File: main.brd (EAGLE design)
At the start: 49.5 x 36.8 mm, 27 parts, among them IC1 FT232RL, U1 ATMEGA328P_TQFP, Y3 16MHz

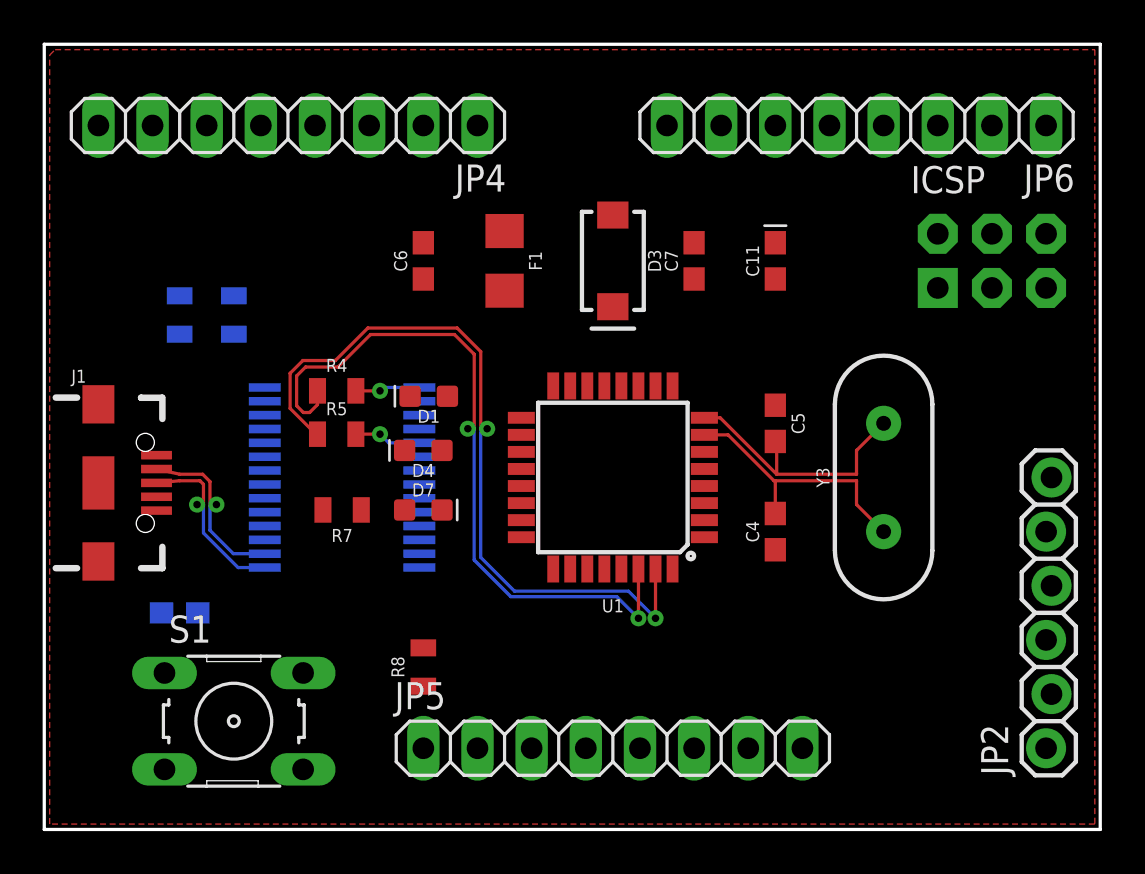
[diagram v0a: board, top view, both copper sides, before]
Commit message: Autorouted
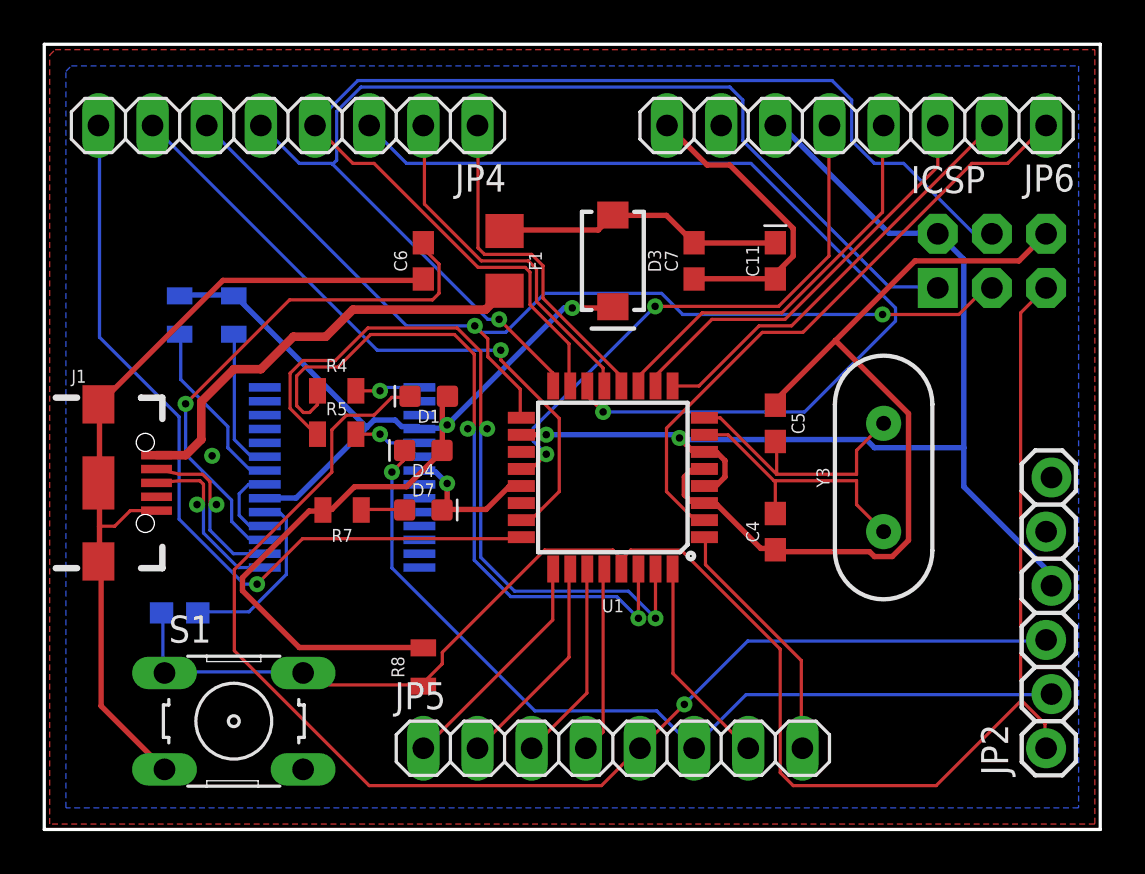
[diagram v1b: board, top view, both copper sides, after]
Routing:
- net GND: track 0.00 -> 105.6 mm, vias 0 -> 2
- net RST: track 0.00 -> 80.1 mm
- net RX: track 0.00 -> 60.1 mm, vias 0 -> 1
- net 5V: track 0.00 -> 56.7 mm, vias 0 -> 2
- net MOSI: track 0.00 -> 55.9 mm
- net MISO: track 0.00 -> 55.4 mm, vias 0 -> 1
- net VCC: track 0.00 -> 54.0 mm, vias 0 -> 2
- net SCK: track 0.00 -> 47.8 mm, vias 0 -> 2
- net PB2: track 0.00 -> 45.9 mm, vias 0 -> 1
- net TX: track 0.00 -> 41.3 mm, vias 0 -> 1
- net PC1: track 0.00 -> 38.3 mm, vias 0 -> 1
- net PC0: track 0.00 -> 30.8 mm, vias 0 -> 1
- net PD4: track 0.00 -> 29.0 mm
- net AREF: track 0.00 -> 26.3 mm, vias 0 -> 2
- net 3.3V: track 0.00 -> 25.1 mm, vias 0 -> 1
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- added copper zone on layer 1, net GND
- added copper zone on layer 16, net GND
- removed copper zone on layer 1, net N$1
